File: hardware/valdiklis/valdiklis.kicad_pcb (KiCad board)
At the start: 2 copper layers, 59 x 67 mm, 4 parts, among them M1 unicon_v1, U1 DHT11, U2 L298HN, U3 DHT11

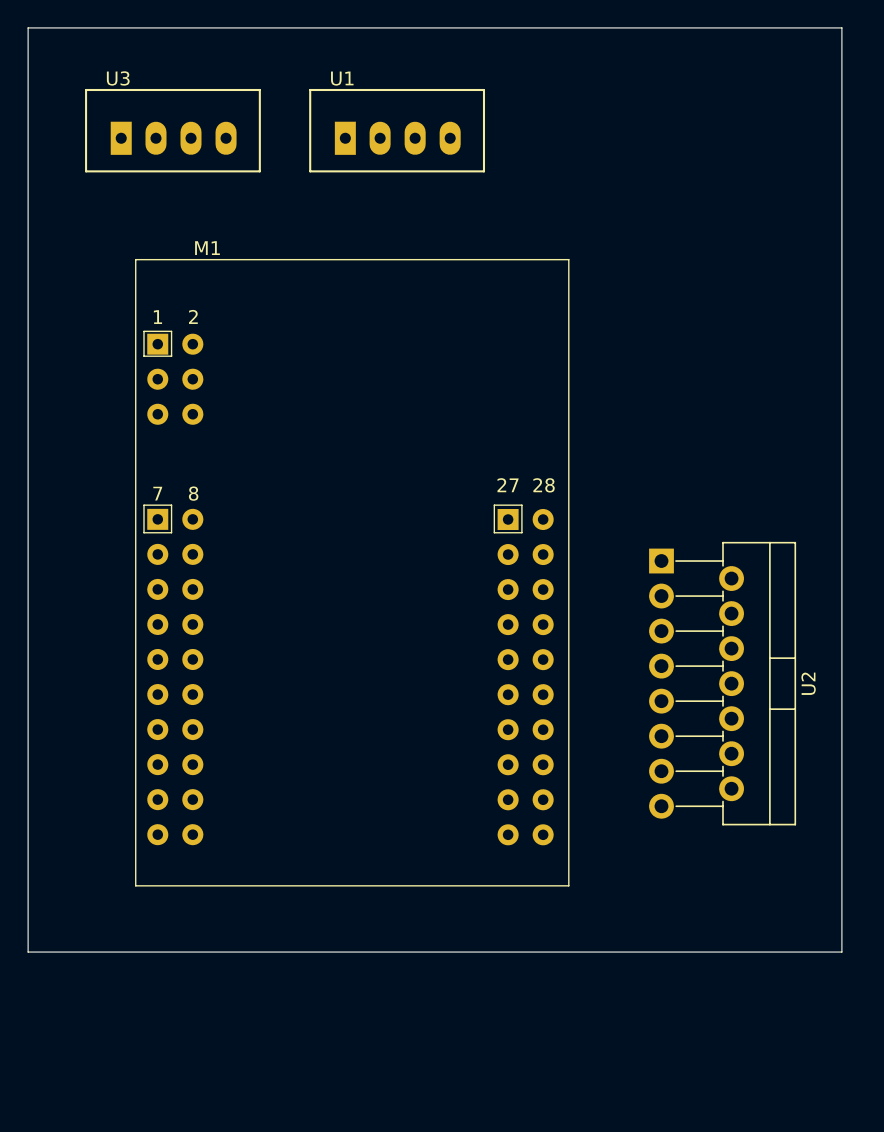
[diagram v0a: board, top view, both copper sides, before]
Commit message: pcb plokstes ir schemos paruosimas
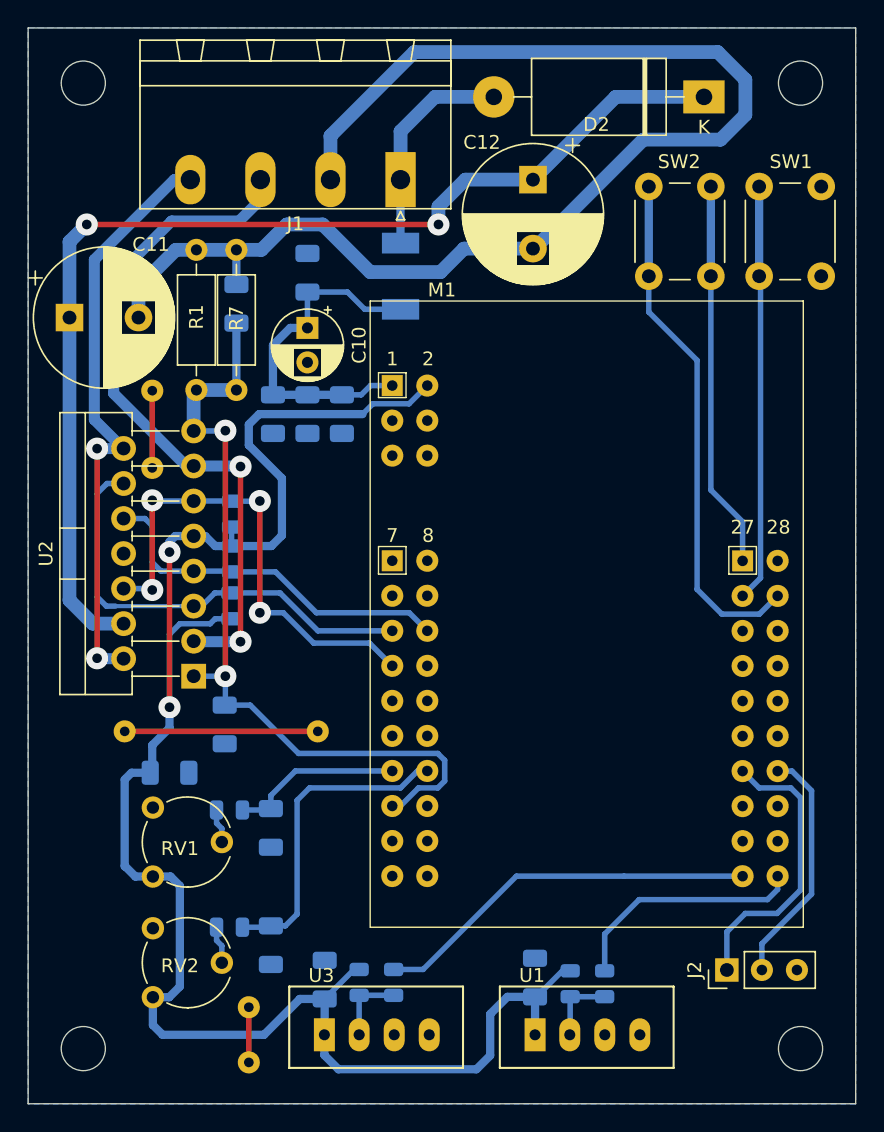
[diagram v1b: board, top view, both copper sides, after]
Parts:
- added C1: 0.1, Capacitor_SMD:C_1206_3216Metric, B.Cu at (107.8, 118.8)
- added C10: CP, Capacitor_THT:CP_Radial_D5.0mm_P2.50mm, F.Cu at (91.2, 71.8)
- added C11: CP, Capacitor_THT:CP_Radial_D10.0mm_P5.00mm, F.Cu at (74.0, 71.0)
- added C12: CP, Capacitor_THT:CP_Radial_D10.0mm_P5.00mm, F.Cu at (107.6, 61.0)
- added C13: 0.1, Capacitor_SMD:C_1206_3216Metric, B.Cu at (86.1, 70.0)
- added C14: 0.1, Capacitor_SMD:C_1206_3216Metric, B.Cu at (85.2, 100.5)
- added C2: 0.1, Capacitor_SMD:C_1206_3216Metric, B.Cu at (88.6, 108.0)
- added C3: 0.1, Capacitor_SMD:C_1206_3216Metric, B.Cu at (88.6, 116.5)
- added C4: 0.1, Capacitor_SMD:C_1206_3216Metric, B.Cu at (92.5, 119.0)
- added C5: 0.1, Capacitor_SMD:C_1206_3216Metric, B.Cu at (93.8, 78.0)
- added C6: 0.1, Capacitor_SMD:C_1206_3216Metric, B.Cu at (91.2, 67.8)
- added C7: 0.1, Capacitor_SMD:C_1206_3216Metric, B.Cu at (91.2, 78.0)
- added C8: 0.1, Capacitor_SMD:C_1206_3216Metric, B.Cu at (81.2, 104.0)
- added C9: 0.1, Capacitor_SMD:C_1206_3216Metric, B.Cu at (88.8, 78.0)
- added D1: D, Diode_SMD:D_MELF, B.Cu at (98.0, 68.0)
- added D2: D, Diode_THT:D_DO-27_P15.24mm_Horizontal, F.Cu at (120.0, 55.0)
- added J1: POWER, Connector_Phoenix_MSTB:PhoenixContact_MSTBA_2,5_4-G-5,08_1x04_P5.08mm_Horizontal, F.Cu at (98.0, 61.0)
- added J2: UART, Connector_PinHeader_2.54mm:PinHeader_1x03_P2.54mm_Vertical, F.Cu at (121.7, 118.3)
- added R1: 1R0, Resistor_THT:R_Axial_DIN0207_L6.3mm_D2.5mm_P10.16mm_Horizontal, F.Cu at (83.2, 76.2)
- added R10: 4,7k, Resistor_SMD:R_0805_2012Metric, B.Cu at (110.3, 119.3)
- added R11: 4,7k, Resistor_SMD:R_0805_2012Metric, B.Cu at (95.0, 119.2)
- added R2: 10k, Resistor_SMD:R_0805_2012Metric, B.Cu at (85.6, 106.7)
- added R3: 10k, Resistor_SMD:R_0805_2012Metric, B.Cu at (85.6, 115.2)
- added R4: 10k, Resistor_SMD:R_0805_2012Metric, B.Cu at (85.8, 85.2)
- added R5: 10k, Resistor_SMD:R_0805_2012Metric, B.Cu at (85.7, 91.9)
- added R6: 10k, Resistor_SMD:R_0805_2012Metric, B.Cu at (85.8, 88.5)
- added R7: 1R0, Resistor_THT:R_Axial_DIN0207_L6.3mm_D2.5mm_P10.16mm_Horizontal, F.Cu at (86.1, 76.2)
- added R8: 47R, Resistor_SMD:R_0805_2012Metric, B.Cu at (112.8, 119.3)
- added R9: 47R, Resistor_SMD:R_0805_2012Metric, B.Cu at (97.5, 119.2)
- added REF**: SolderWirePad_1x01_Drill0.8mm, Connector_Wire:SolderWirePad_1x01_Drill0.8mm, F.Cu at (80.0, 76.3)
- added REF**: SolderWirePad_1x01_Drill0.8mm, Connector_Wire:SolderWirePad_1x01_Drill0.8mm, F.Cu at (78.0, 101.0)
- added REF**: SolderWirePad_1x01_Drill0.8mm, Connector_Wire:SolderWirePad_1x01_Drill0.8mm, F.Cu at (80.0, 81.9)
- added REF**: SolderWirePad_1x01_Drill0.8mm, Connector_Wire:SolderWirePad_1x01_Drill0.8mm, F.Cu at (87.0, 121.0)
- added REF**: SolderWirePad_1x01_Drill0.8mm, Connector_Wire:SolderWirePad_1x01_Drill0.8mm, F.Cu at (87.0, 125.0)
- added REF**: SolderWirePad_1x01_Drill0.8mm, Connector_Wire:SolderWirePad_1x01_Drill0.8mm, F.Cu at (92.0, 101.0)
- added REF**: MountingHole_3.2mm_M3, MountingHole:MountingHole_3.2mm_M3, F.Cu at (75.0, 124.0)
- added REF**: MountingHole_3.2mm_M3, MountingHole:MountingHole_3.2mm_M3, F.Cu at (127.0, 124.0)
- added REF**: MountingHole_3.2mm_M3, MountingHole:MountingHole_3.2mm_M3, F.Cu at (127.0, 54.0)
- added REF**: MountingHole_3.2mm_M3, MountingHole:MountingHole_3.2mm_M3, F.Cu at (75.0, 54.0)
- added RV1: 5k, Potentiometer_THT:Potentiometer_Piher_PT-6-V_Vertical, F.Cu at (80.0, 111.5)
- added RV2: 5k, Potentiometer_THT:Potentiometer_Piher_PT-6-V_Vertical, F.Cu at (80.0, 120.3)
- added SW1: RESET, Button_Switch_THT:SW_PUSH_6mm_H5mm, F.Cu at (124.0, 68.0)
- added SW2: RESET, Button_Switch_THT:SW_PUSH_6mm_H5mm, F.Cu at (116.0, 68.0)
- M1: value unicon_v1 -> UniCon
- moved U3 66.6 mm to (93.7, 123.0)
- moved U1 66.4 mm to (109.0, 123.0)
- moved U2 34.9 mm to (83.0, 97.0), turned to 90 degrees
- moved M1 17.3 mm to (96.0, 115.0)
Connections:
- M1 pad 1: /12VDC -> /12V1
- M1 pad 11: Net-(M1-Pad11) -> /L298_IN1
- M1 pad 12: Net-(M1-Pad12) -> /L298_IN2
- M1 pad 13: Net-(M1-Pad13) -> /L298_ENA
- M1 pad 19: Net-(M1-Pad19) -> /AD1
- M1 pad 2: /5VDC -> +5V
- M1 pad 20: Net-(M1-Pad20) -> /AD2
- M1 pad 21: Net-(M1-Pad21) -> /ADC
- M1 pad 27: Net-(M1-Pad27) -> /3VDC
- M1 pad 29: Net-(M1-Pad29) -> /~RST
- M1 pad 30: Net-(M1-Pad30) -> /BOOT
- M1 pad 39: Net-(M1-Pad39) -> /UART_TX
- M1 pad 40: Net-(M1-Pad40) -> /UART_RX
- M1 pad 45: Net-(M1-Pad45) -> /DHT1
- M1 pad 46: Net-(M1-Pad46) -> /DHT2
- U1 pad 2: /DHT1 -> Net-(R10-Pad1)
- U2 pad 1: Net-(R1-Pad1) -> /ADC
- U2 pad 10: /IN1 -> /L298_IN2
- U2 pad 11: /ENA -> /L298_ENA
- U2 pad 12: /IN2 -> /L298_IN1
- U2 pad 13: /MOTA -> /MOTB
- U2 pad 14: /MOTB -> /MOTA
- U2 pad 15: Net-(R1-Pad1) -> /ADC
- U2 pad 5: /IN1 -> /L298_IN1
- U2 pad 6: /ENA -> /L298_ENA
- U2 pad 7: /IN2 -> /L298_IN2
- U2 pad 9: /5VDC -> +5V
- U3 pad 2: /DHT2 -> Net-(R11-Pad1)
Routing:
- net +5V: track 0.00 -> 132.9 mm, vias 0 -> 2
- net /GND1: track 0.00 -> 95.9 mm
- net /12VDC: track 0.00 -> 81.7 mm, vias 0 -> 2
- net /ADC: track 0.00 -> 58.9 mm, vias 0 -> 2
- net /MOTB: track 0.00 -> 50.3 mm, vias 0 -> 2
- net /MOTA: track 0.00 -> 43.0 mm, vias 0 -> 2
- net /BOOT: track 0.00 -> 37.8 mm
- net /L298_ENA: track 0.00 -> 35.7 mm, vias 0 -> 4
- net /L298_IN1: track 0.00 -> 32.9 mm
- net /~RST: track 0.00 -> 30.3 mm
- net /DHT1: track 0.00 -> 28.1 mm
- net /3VDC: track 0.00 -> 28.1 mm
- net /L298_IN2: track 0.00 -> 26.9 mm
- net /12V1: track 0.00 -> 25.4 mm
- net GND: track 0.00 -> 23.6 mm
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- added copper zone on B.Cu, net GND
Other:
- board size 59 x 67 mm -> 60 x 78 mm
- net class power added: clearance 0.4, trace_width 0.6, via_dia 1.6, via_drill 0.7
